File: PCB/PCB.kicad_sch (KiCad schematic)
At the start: 0 parts

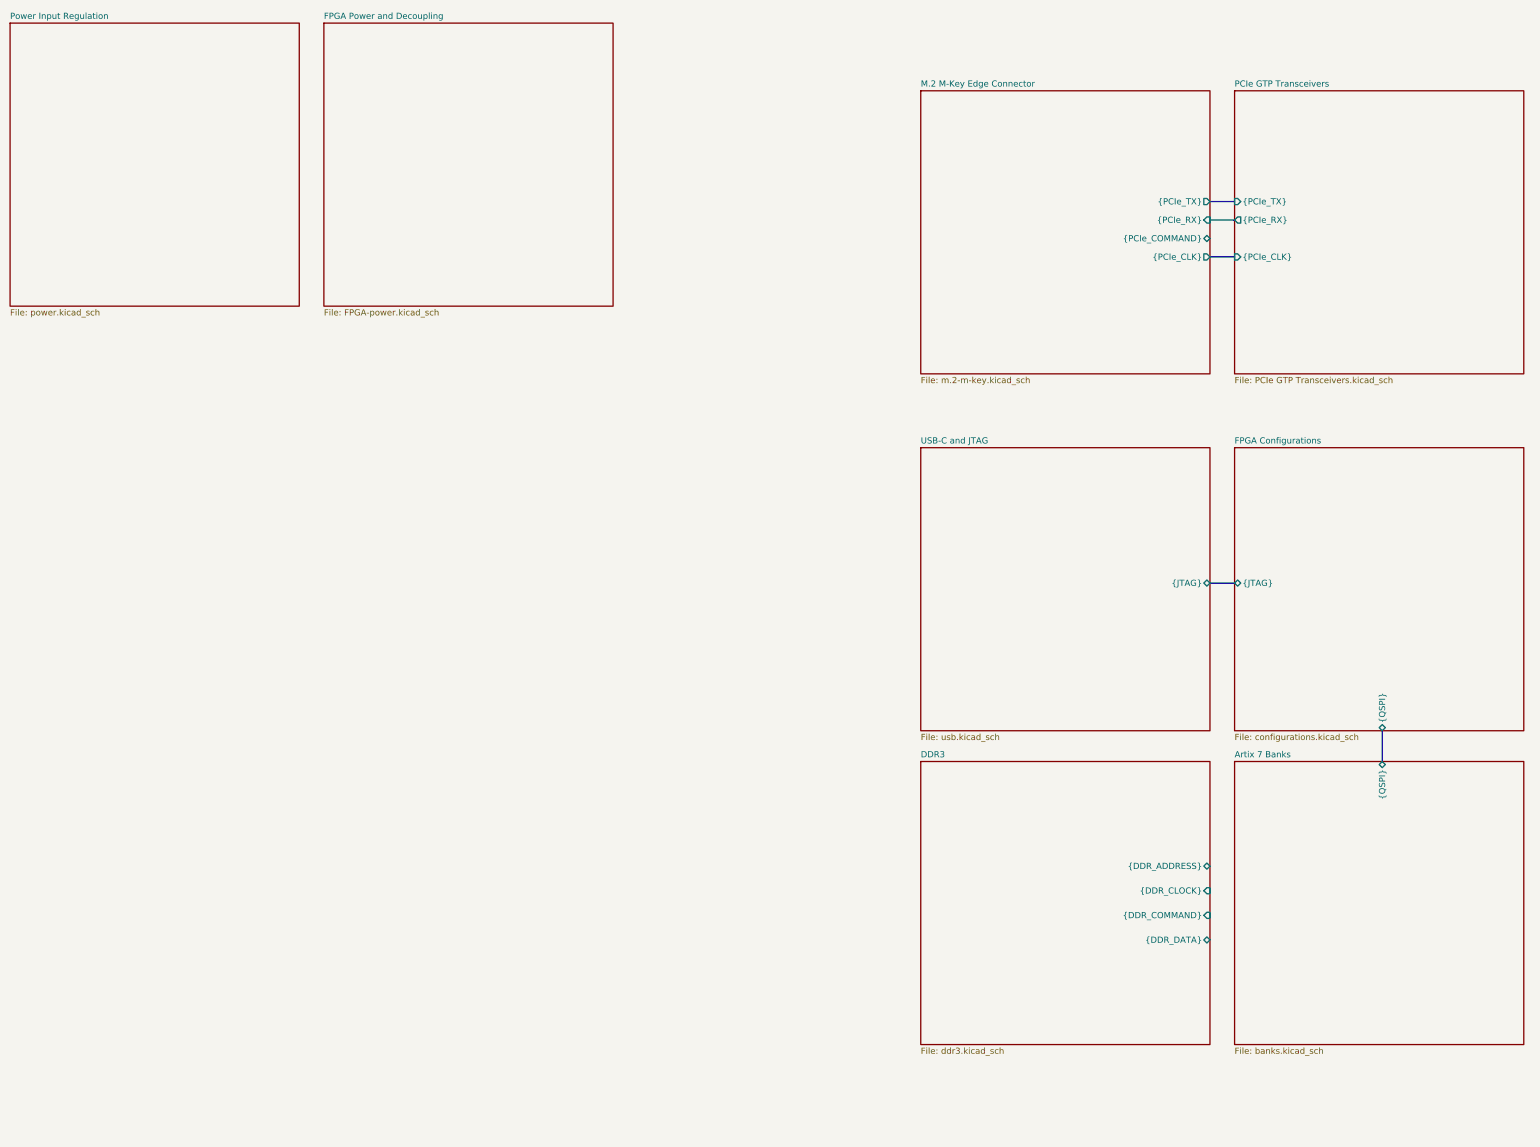
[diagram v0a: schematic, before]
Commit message: cleaning up the schematic some more, getting ready to wire the clocks, HDMI and ethernet!
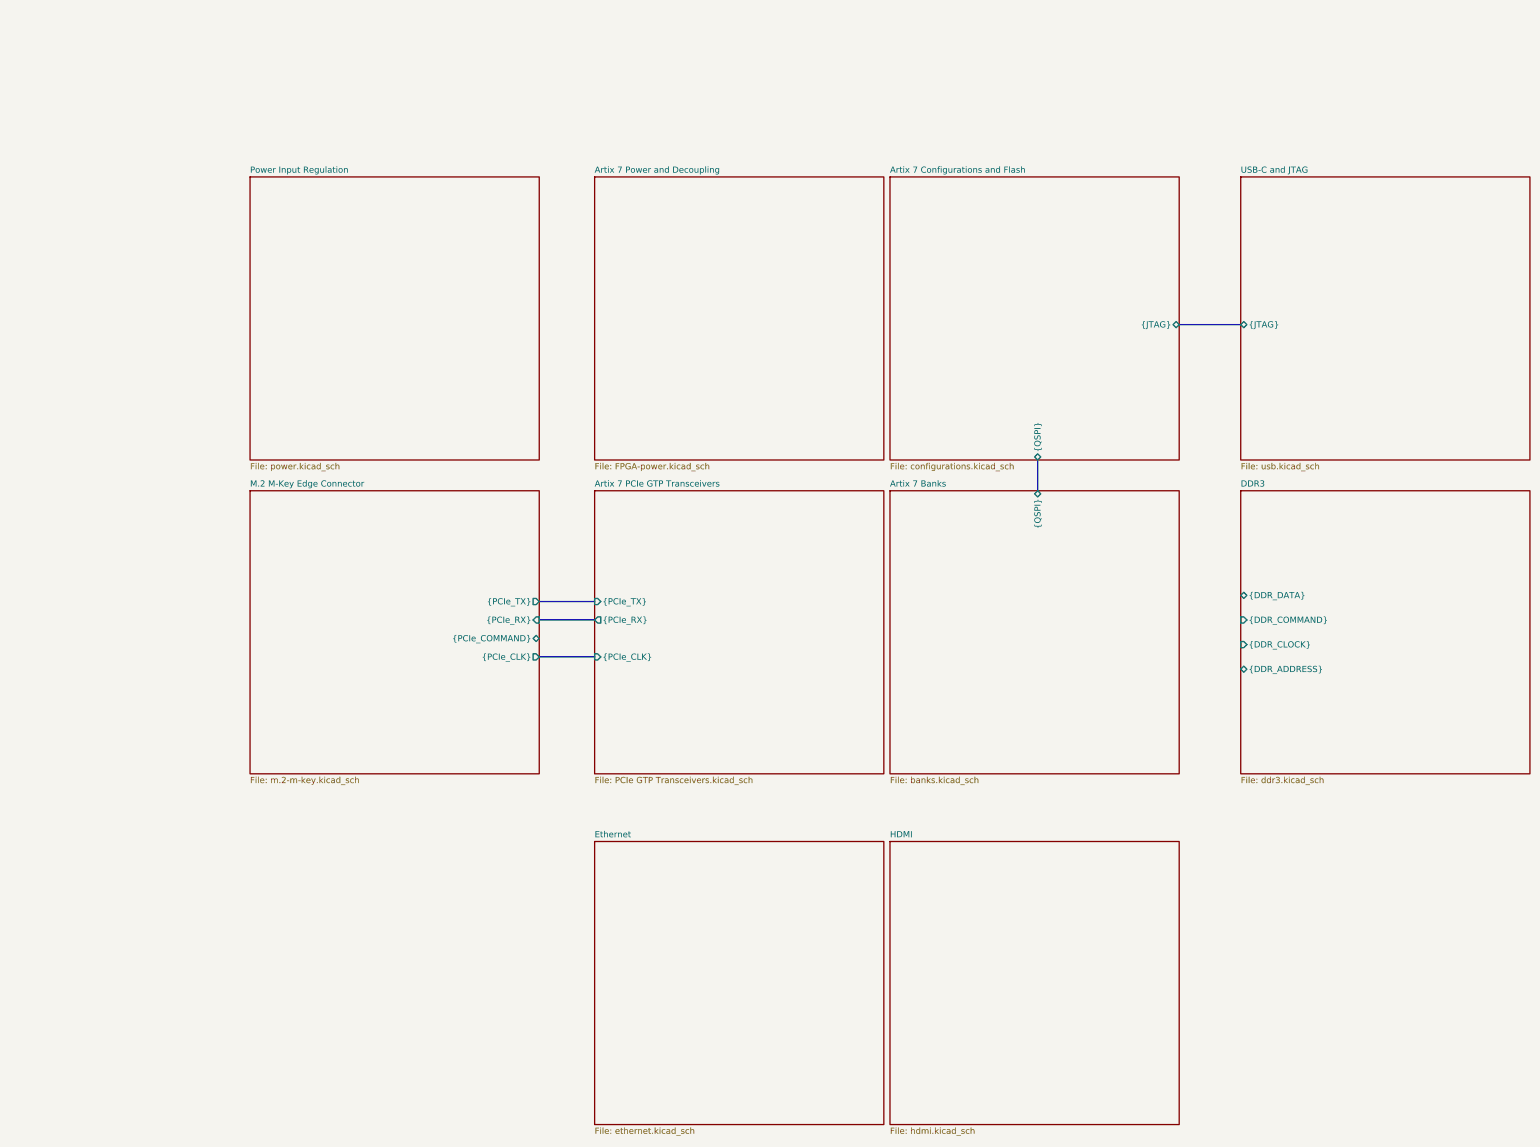
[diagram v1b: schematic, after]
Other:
- sheet FPGA Configurations renamed Artix 7 Configurations and Flash
- sheet FPGA Power and Decoupling renamed Artix 7 Power and Decoupling
- sheet PCIe GTP Transceivers renamed Artix 7 PCIe GTP Transceivers
- added sheet Ethernet (ethernet.kicad_sch)
- added sheet HDMI (hdmi.kicad_sch)
